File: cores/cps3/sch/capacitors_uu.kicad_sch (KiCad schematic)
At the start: 131 parts, among them U1 7400, U2 74LS08, U4 7400

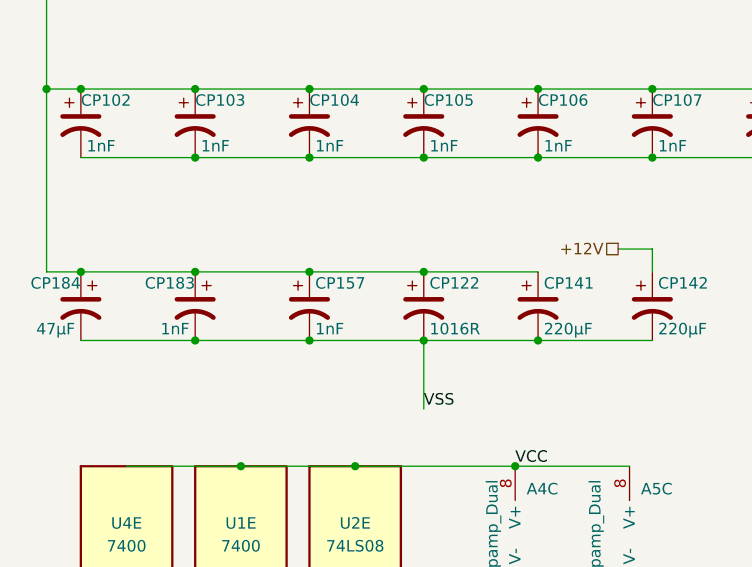
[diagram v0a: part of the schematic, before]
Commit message: wip_cre_cps3
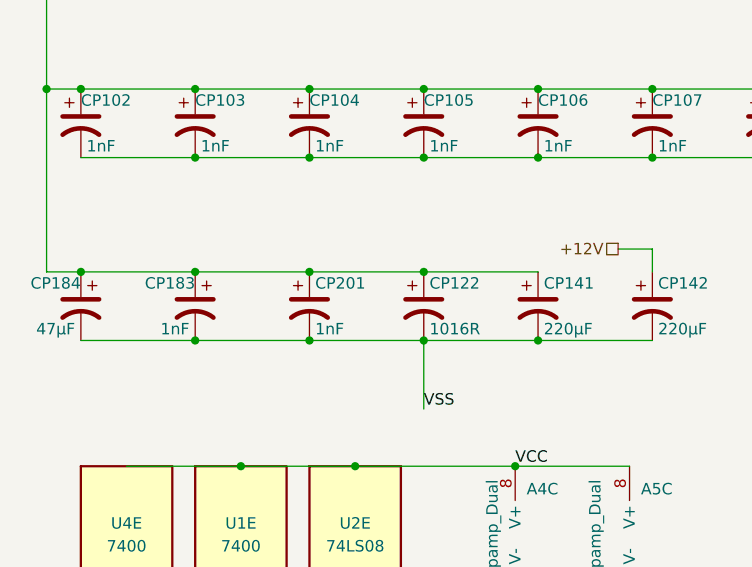
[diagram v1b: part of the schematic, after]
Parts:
- renumbered CP157 to CP201
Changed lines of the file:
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@@
   (symbol (lib_id "Device:C_Polarized_US") (at 114.3 195.58 0) (unit 1)
     (in_bom yes) (on_board yes)
-    (property "Reference" "CP157" (id 0) (at 114.935 193.04 0)
+    (property "Reference" "CP201" (id 0) (at 114.935 193.04 0)
       (effects (font (size 1.27 1.27)) (justify left))
     )
